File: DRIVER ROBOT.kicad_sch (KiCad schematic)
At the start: 9 parts, among them J1 INPUT 12V, J2 OUT MOTOR 1, J3 OUT MOTOR 2, J4 OLED 3 INCH

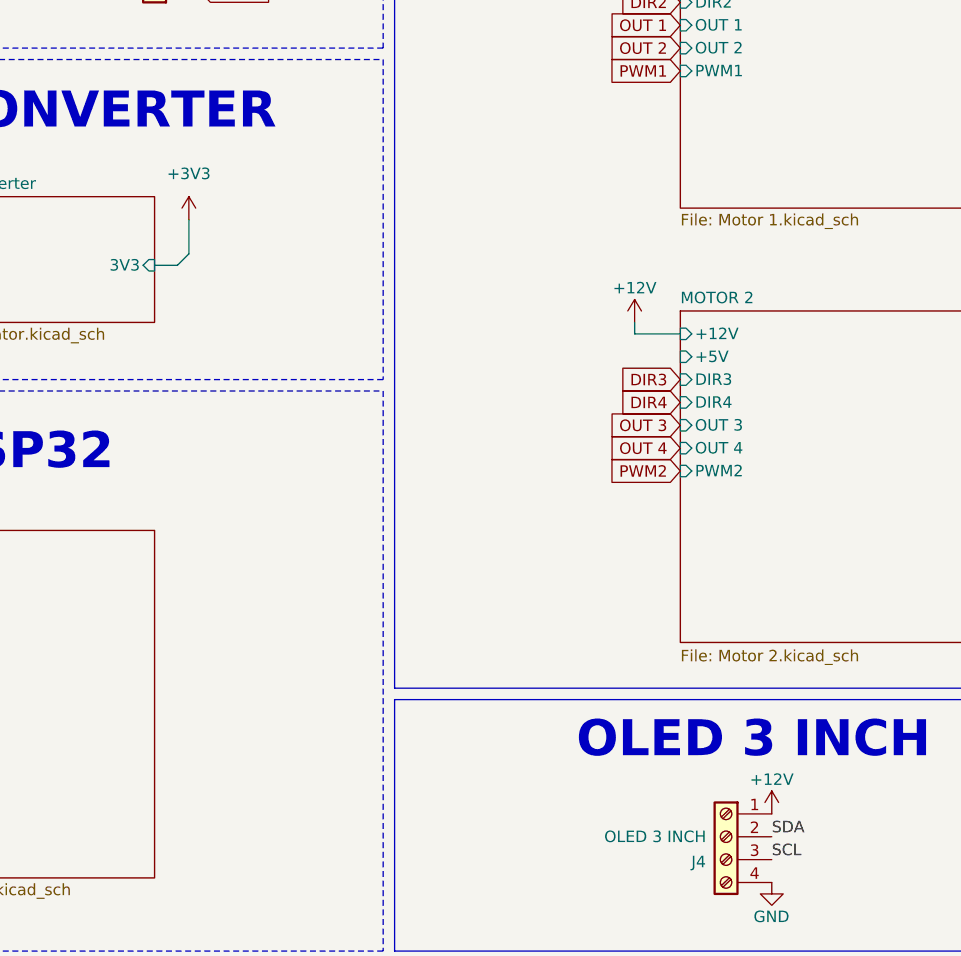
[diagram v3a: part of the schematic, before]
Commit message: layout v2
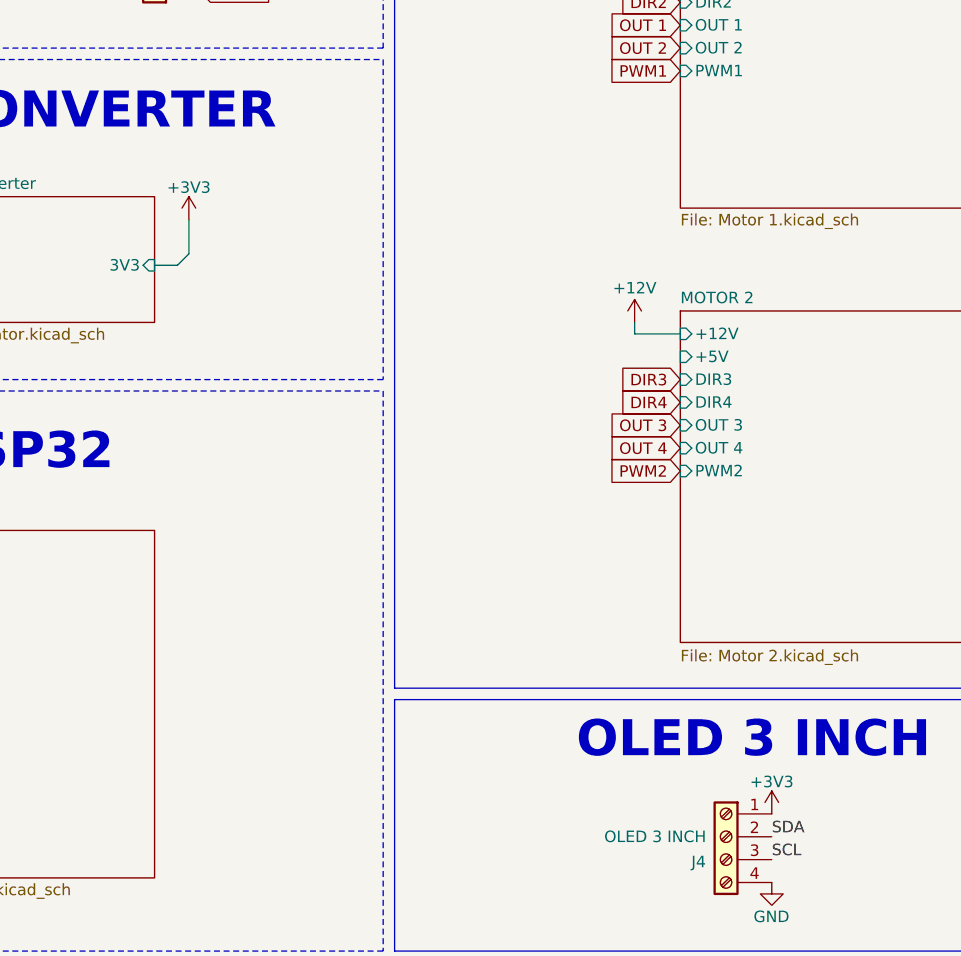
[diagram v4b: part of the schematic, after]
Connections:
- net +12V: no longer J4.1 (Pin_1)
- net +3V3: now also J4.1 (Pin_1)
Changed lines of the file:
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@@
-	(symbol
-		(lib_id "power:+12V")
-		(at 189.23 140.97 0)
-		(unit 1)
-		(body_style 1)
-		(exclude_from_sim no)
-		(in_bom yes)
-		(on_board yes)
-		(in_pos_files yes)
-		(dnp no)
-		(property "Reference" "#PWR055"
-			(at 189.23 144.78 0)
-			(hide yes)
-			(show_name no)
-			(do_not_autoplace no)
-			(effects
-				(font
-					(size 1.27 1.27)
-				)
-			)
-		)
-		(property "Value" "+12V"
-			(at 189.23 137.16 0)
-			(show_name no)
-			(do_not_autoplace no)
-			(effects
-				(font
-					(size 1.27 1.27)
-				)
-			)
-		)
-		(property "Footprint" ""
-			(at 189.23 140.97 0)
-			(hide yes)
-			(show_name no)
-			(do_not_autoplace no)
-			(effects
-				(font
-					(size 1.27 1.27)
-				)
-			)
-		)
-		(property "Datasheet" ""
-			(at 189.23 140.97 0)
-			(hide yes)
-			(show_name no)
-			(do_not_autoplace no)
-			(effects
-				(font
-					(size 1.27 1.27)
-				)
-			)
-		)
-		(property "Description" "Power symbol creates a global label with name \"+12V\""
-			(at 189.23 140.97 0)
-			(hide yes)
-			(show_name no)
-			(do_not_autoplace no)
-			(effects
-				(font
-					(size 1.27 1.27)
-				)
-			)
-		)
-		(pin "1"
-		)
-		(instances
-			(project "DRIVER ROBOT"
-				(path "/b1fe2535-19ad-46cf-8d17-623aba53d479"
-					(reference "#PWR055")
-					(unit 1)
-				)
-			)
-		)
-	)
 	(symbol
 		(lib_id "power:+12V")
@@
 		(in_pos_files yes)
 		(dnp no)
-		(fields_autoplaced yes)
 		(property "Reference" "#PWR049"
 			(at 124.46 78.74 0)
@@
 		)
 		(property "Value" "+3V3"
-			(at 124.46 69.85 0)
+			(at 124.46 71.374 0)
 			(show_name no)
 			(do_not_autoplace no)
@@
 					(unit 1)
 				)
+			)
+		)
+	)
+	(symbol
+		(lib_id "power:+3V3")
+		(at 189.23 140.97 0)
+		(unit 1)
+		(body_style 1)
+		(exclude_from_sim no)
+		(in_bom yes)
+		(on_board yes)
+		(in_pos_files yes)
+		(dnp no)
+		(property "Reference" "#PWR055"
+			(at 189.23 144.78 0)
+			(hide yes)
+			(show_name no)
+			(do_not_autoplace no)
+			(effects
+				(font
+					(size 1.27 1.27)
+				)
+			)
+		)
+		(property "Value" "+3V3"
+			(at 189.23 137.414 0)
+			(show_name no)
+			(do_not_autoplace no)
+			(effects
+				(font
+					(size 1.27 1.27)
+				)
+			)
+		)
+		(property "Footprint" ""
+			(at 189.23 140.97 0)
+			(hide yes)
+			(show_name no)
+			(do_not_autoplace no)
+			(effects
+				(font
+					(size 1.27 1.27)
+				)
+			)
+		)
+		(property "Datasheet" ""
+			(at 189.23 140.97 0)
+			(hide yes)
+			(show_name no)
+			(do_not_autoplace no)
+			(effects
+				(font
+					(size 1.27 1.27)
+				)
+			)
+		)
+		(property "Description" "Power symbol creates a global label with name \"+3V3\""
+			(at 189.23 140.97 0)
+			(hide yes)
+			(show_name no)
+			(do_not_autoplace no)
+			(effects
+				(font
+					(size 1.27 1.27)
+				)
+			)
+		)
+		(pin "1"
+		)
+		(instances
+			(project "DRIVER ROBOT"
+				(path "/b1fe2535-19ad-46cf-8d17-623aba53d479"
+					(reference "#PWR055")
+					(unit 1)
+				)
